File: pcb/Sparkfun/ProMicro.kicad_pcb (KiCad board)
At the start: 2 copper layers, 22 parts, among them J1 Conn_01x02, U2 MCP3x61/NC, U3 TLV75533PDRV, U4 MCP1501-33xRW

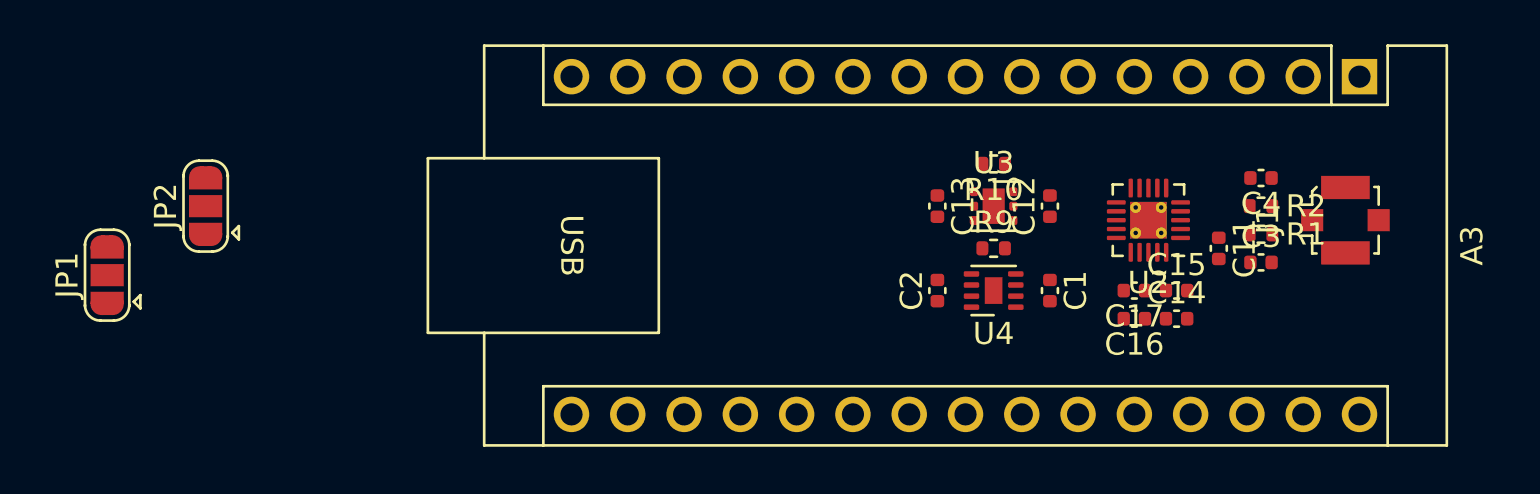
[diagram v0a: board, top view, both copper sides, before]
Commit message: update pcbs
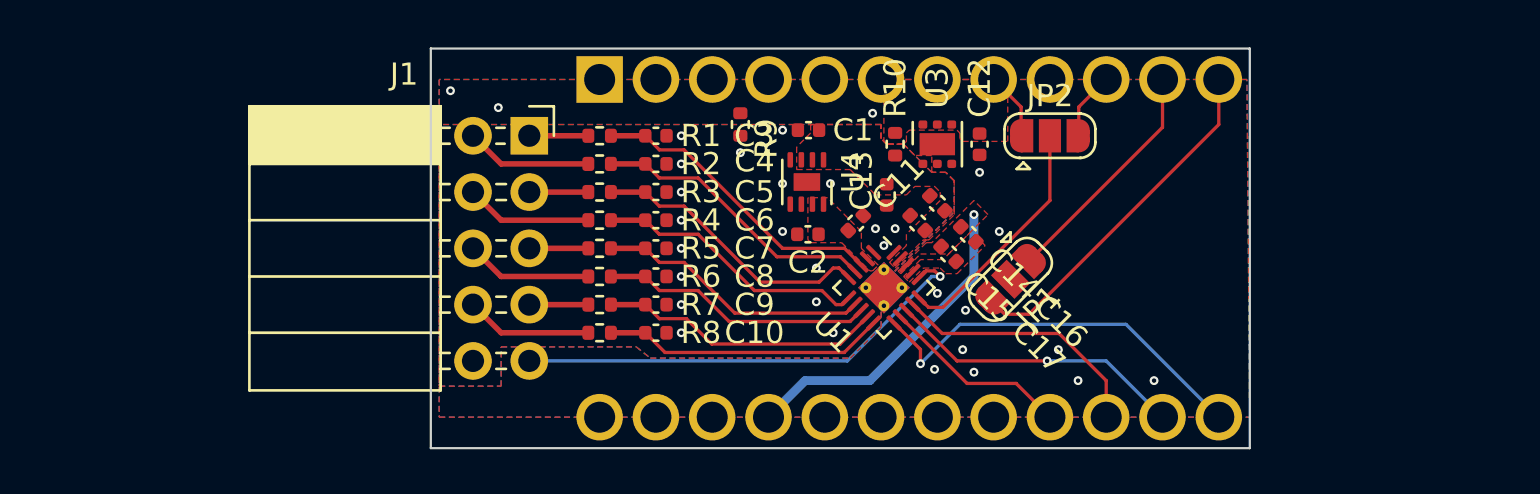
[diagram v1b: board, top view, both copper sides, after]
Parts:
- removed U2: MCP3x61/NC, Package_DFN_QFN:QFN-20-1EP_3x3mm_P0.4mm_EP1.65x1.65mm_ThermalVias
- added C10: 10p, Capacitor_SMD:C_0402_1005Metric, F.Cu at (118.1, 97.8)
- added C5: 10p, Capacitor_SMD:C_0402_1005Metric, F.Cu at (118.1, 91.4)
- added C6: 10p, Capacitor_SMD:C_0402_1005Metric, F.Cu at (118.1, 92.7)
- added C7: 10p, Capacitor_SMD:C_0402_1005Metric, F.Cu at (118.1, 94.0)
- added C8: 10p, Capacitor_SMD:C_0402_1005Metric, F.Cu at (118.1, 95.2)
- added C9: 10p, Capacitor_SMD:C_0402_1005Metric, F.Cu at (118.1, 96.5)
- added R3: 1k, Resistor_SMD:R_0402_1005Metric, F.Cu at (115.6, 91.4)
- added R4: 1k, Resistor_SMD:R_0402_1005Metric, F.Cu at (115.6, 92.7)
- added R5: 1k, Resistor_SMD:R_0402_1005Metric, F.Cu at (115.6, 94.0)
- added R6: 1k, Resistor_SMD:R_0402_1005Metric, F.Cu at (115.6, 95.2)
- added R7: 1k, Resistor_SMD:R_0402_1005Metric, F.Cu at (115.6, 96.5)
- added R8: 1k, Resistor_SMD:R_0402_1005Metric, F.Cu at (115.6, 97.8)
- added U1: MCP3x64/NC, Package_DFN_QFN:QFN-20-1EP_3x3mm_P0.4mm_EP1.65x1.65mm_ThermalVias, F.Cu at (128.4, 95.8)
- A3: footprint Module:Arduino_Nano -> pcb:ProMicro; moved to B.Cu
- J1: value Conn_01x02 -> Conn_02x05_Odd_Even; footprint Connector_Coaxial:U.FL_Molex_MCRF_73412-0110_Vertical -> Connector_PinSocket_2.54mm:PinSocket_2x05_P2.54mm_Horizontal
- U4: value MCP1501-33xRW -> MCP1501-30xRW
- moved JP1 40.8 mm to (134.1, 95.4), turned to -135 degrees
- moved JP2 38.2 mm to (135.9, 88.9), turned to 0 degrees
- moved J1 37.0 mm to (112.4, 88.9), turned to 0 degrees
- moved A3 34.3 mm to (115.6, 86.4)
- moved R1 30.2 mm to (115.6, 88.9), turned to 0 degrees
- moved R2 29.9 mm to (115.6, 90.2), turned to 0 degrees
- moved C3 27.9 mm to (118.1, 88.9)
- moved C4 27.3 mm to (118.1, 90.2)
- moved C11 16.4 mm to (127.1, 92.8), turned to 45 degrees
- moved C1 13.1 mm to (125.0, 88.6), turned to 180 degrees
- moved R9 12.7 mm to (121.9, 88.4), turned to -90 degrees
- moved C15 12.1 mm to (129.9, 92.8), turned to 135 degrees
- moved C14 12.0 mm to (130.8, 91.9), turned to 135 degrees
- moved U4 9.75 mm to (124.9, 91.0), turned to -90 degrees
- moved C17 8.54 mm to (131.3, 94.2), turned to -45 degrees
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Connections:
- net Net-(J1-Pin_1) renamed /CH0
- net Net-(J1-Pin_2) renamed /CH1
- net Net-(U2-VREF+) renamed /VREF+
- A3 pad 13: unconnected-(A3-CS/D10-Pad13) -> /SS
- A3 pad 21: +5V -> VDD
- A3 pad 24: unconnected-(A3-RAW-Pad24) -> +5V
- A3 pad 9: /SS -> unconnected-(A3-D6/A7-Pad9)
- U4 pad 9: (no net) -> GNDA
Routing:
- net /MCLK: track 0.00 -> 21.3 mm, vias 0 -> 1
- net /SS: track 0.00 -> 18.3 mm, vias 0 -> 1
- net Net-(A3-D9/A9): track 0.00 -> 16.2 mm
- net VDD: track 0.00 -> 14.7 mm, vias 0 -> 1
- net Net-(U1-CH0): track 0.00 -> 13.7 mm
- net /MOSI: track 0.00 -> 13.5 mm, vias 0 -> 1
- net Net-(U1-CH1): track 0.00 -> 13.0 mm
- net Net-(U1-CH2): track 0.00 -> 12.9 mm
- net Net-(U1-CH6): track 0.00 -> 12.8 mm
- net Net-(U1-CH7): track 0.00 -> 12.8 mm
- net Net-(U1-CH3): track 0.00 -> 12.4 mm
- net Net-(U1-CH4): track 0.00 -> 12.4 mm
- net Net-(U1-CH5): track 0.00 -> 12.3 mm
- net /MISO: track 0.00 -> 11.8 mm
- net /IRQ: track 0.00 -> 11.0 mm
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- added copper zone on F.Cu, net +5V
- added copper zone on F.Cu, net /VREF+
- added copper zone on B.Cu, net GNDA
- added copper zone on F.Cu, net GNDA
- added copper zone on B.Cu, net GNDD
- added copper zone on F.Cu, net GNDD
- added copper zone on F.Cu, net VDD
- added copper zone on F.Cu, net VDDA
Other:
- board outline added: 37 x 18 mm
